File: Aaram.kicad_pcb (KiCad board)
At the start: 2 copper layers, 100 x 100 mm, 52 parts, among them J1 Conn_01x03, J2 Conn_01x02, J3 AC_OUT, J4 SWITCH_IN, J5 5V_OUT, J6 PSU_AC_IN, J8 SPARE_PINS, K1 10A cube relay, K2 10A cube relay, K3 10A cube relay, Q1 BT136-600, Q2 2N2222A, Q3 2N2222A, Q4 2N2222A, U1 ESP32-DevKitC, U2 TLP281-4GB_F_

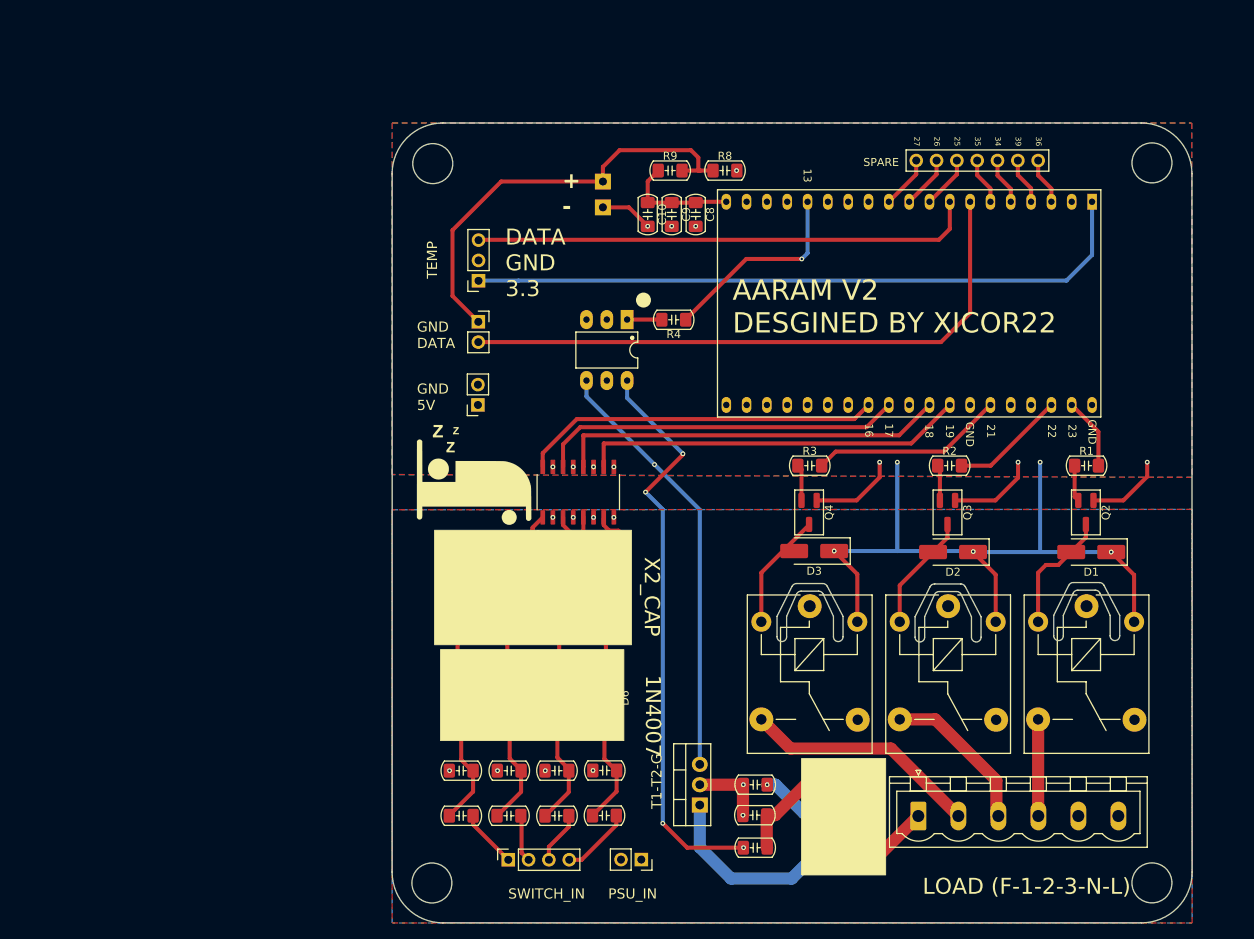
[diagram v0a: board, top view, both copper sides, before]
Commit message: Updated mostly everything
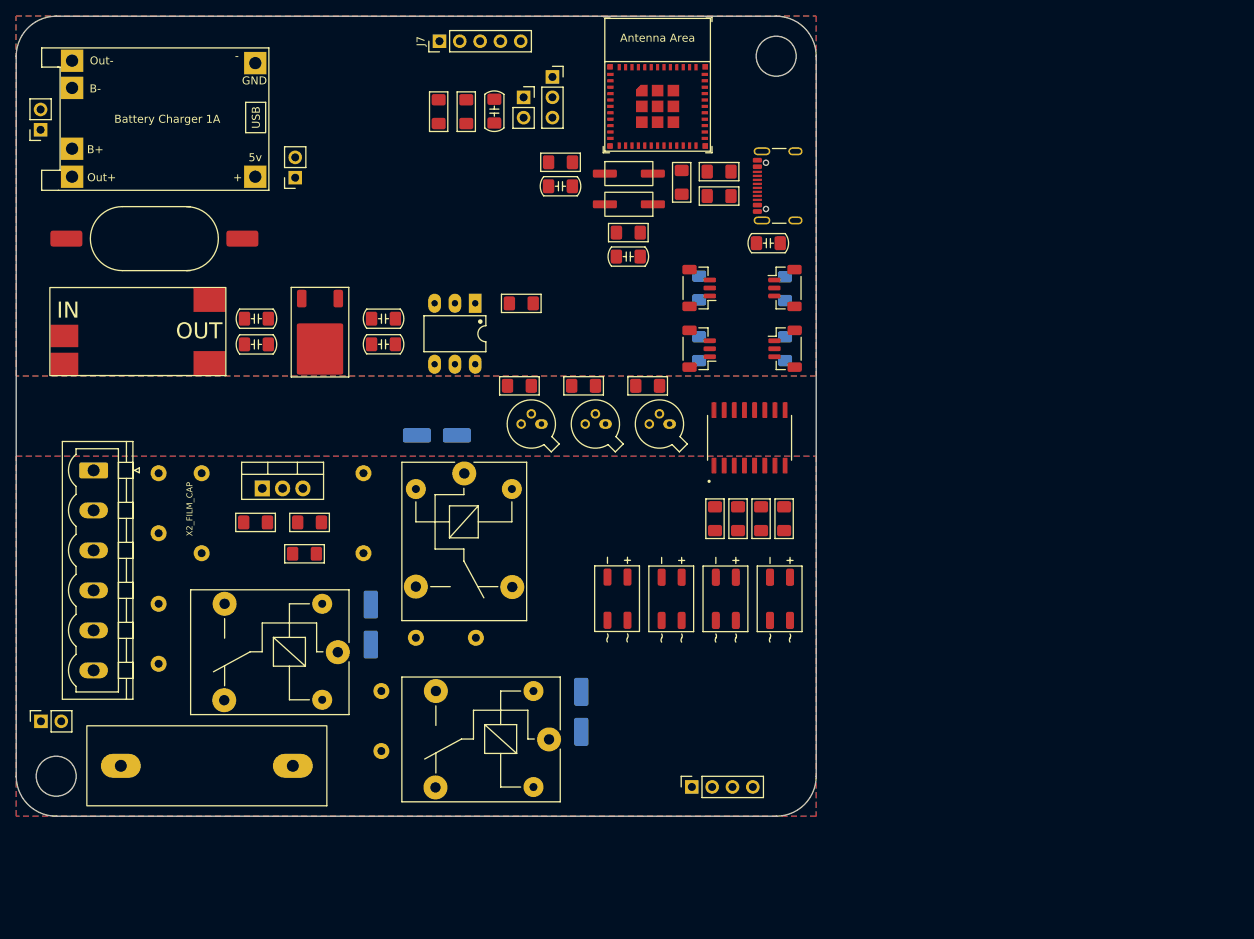
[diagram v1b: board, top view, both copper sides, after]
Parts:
- removed C10, C8, C9: 22uf, PCM_Capacitor_SMD_Handsoldering_AKL:C_1206_3216Metric_Pad1.42x1.75mm
- removed C3, C5: CP_Axial_L10.0mm_D4.5mm_P15.00mm, Xicor_Custom stuff:Axial_Capacitor_P10mm_W4.5mm
- removed D4, D5, D6, D7: 1N4007, Diode_SMD:D_SMA_Handsoldering
- removed G***: LOGO, LOGO
- removed R11, R13: 10K, PCM_Capacitor_SMD_Handsoldering_AKL:C_1206_3216Metric_Pad1.42x1.75mm
- removed R16: 1M, PCM_Capacitor_SMD_Handsoldering_AKL:C_1206_3216Metric_Pad1.42x1.75mm
- added C11: 10uf, PCM_Capacitor_SMD_Handsoldering_AKL:C_1206_3216Metric_Pad1.42x1.75mm, F.Cu at (65.6, 57.4)
- added C12: 10uf, PCM_Capacitor_SMD_Handsoldering_AKL:C_1206_3216Metric_Pad1.42x1.75mm, F.Cu at (65.6, 60.6)
- added C16: 1uf, PCM_Capacitor_SMD_Handsoldering_AKL:C_1206_3216Metric_Pad1.42x1.75mm, F.Cu at (113.7, 47.9)
- added C18: 0.1uf, PCM_Capacitor_SMD_Handsoldering_AKL:C_1206_3216Metric_Pad1.42x1.75mm, F.Cu at (87.7, 40.8)
- added C19: 0.1uf, PCM_Capacitor_SMD_Handsoldering_AKL:C_1206_3216Metric_Pad1.42x1.75mm, F.Cu at (96.2, 49.6)
- added D10: MB6S, PCM_Diode_SMD_AKL:Diode_Bridge_MBS, F.Cu at (108.4, 92.4)
- added D11: MB6S, PCM_Diode_SMD_AKL:Diode_Bridge_MBS, F.Cu at (115.1, 92.4)
- added D8: MB6S, PCM_Diode_SMD_AKL:Diode_Bridge_MBS, F.Cu at (94.8, 92.4)
- added D9: MB6S, PCM_Diode_SMD_AKL:Diode_Bridge_MBS, F.Cu at (101.6, 92.4)
- added F1: Fuse, Xicor_Custom stuff:BLX-A, F.Cu at (43.5, 113.3)
- added J10: Conn_01x03_Socket, Connector_JST:JST_SH_BM03B-SRSS-TB_1x03-1MP_P1.00mm_Vertical, F.Cu at (115.8, 61.1)
- added J11: Conn_01x03_Socket, Connector_JST:JST_SH_BM03B-SRSS-TB_1x03-1MP_P1.00mm_Vertical, F.Cu at (105.1, 61.1)
- added J12: Conn_01x03_Socket, Connector_JST:JST_SH_BM03B-SRSS-TB_1x03-1MP_P1.00mm_Vertical, F.Cu at (105.1, 53.5)
- added J13: Conn_01x03_Socket, Connector_JST:JST_SH_BM03B-SRSS-TB_1x03-1MP_P1.00mm_Vertical, F.Cu at (115.8, 53.5)
- added J7: Conn_01x05, Connector_PinHeader_2.54mm:PinHeader_1x05_P2.54mm_Vertical, F.Cu at (72.6, 22.7)
- added J9: Conn_01x02, Connector_PinSocket_2.54mm:PinSocket_1x02_P2.54mm_Vertical, F.Cu at (22.8, 33.8)
- added R19: 100K, PCM_Resistor_SMD_AKL:R_1206_3216Metric_Pad1.42x1.75mm_HandSolder, F.Cu at (115.7, 82.4)
- added R20: 10K, PCM_Resistor_SMD_AKL:R_1206_3216Metric_Pad1.42x1.75mm_HandSolder, B.Cu at (115.8, 53.6)
- added R21: 10k, PCM_Resistor_SMD_AKL:R_1206_3216Metric_Pad1.42x1.75mm_HandSolder, F.Cu at (96.2, 46.6)
- added R22: 10k, PCM_Resistor_SMD_AKL:R_1206_3216Metric_Pad1.42x1.75mm_HandSolder, F.Cu at (102.9, 40.3)
- added R23: 100K, PCM_Resistor_SMD_AKL:R_1206_3216Metric_Pad1.42x1.75mm_HandSolder, F.Cu at (107.1, 82.4)
- added R25: 10K, PCM_Resistor_SMD_AKL:R_1206_3216Metric_Pad1.42x1.75mm_HandSolder, B.Cu at (105.1, 53.5)
- added R26: 10K, PCM_Resistor_SMD_AKL:R_1206_3216Metric_Pad1.42x1.75mm_HandSolder, B.Cu at (105.1, 61.1)
- added R27: 10K, PCM_Resistor_SMD_AKL:R_1206_3216Metric_Pad1.42x1.75mm_HandSolder, B.Cu at (115.8, 61.1)
- added RV1: Varistor, Xicor_Custom stuff:Varistor_10D431K, F.Cu at (37.5, 93.0)
- added RV2: Varistor, Xicor_Custom stuff:Varistor_10D431K, F.Cu at (69.7, 97.3)
- added RV3: Varistor, Xicor_Custom stuff:Varistor_10D431K, F.Cu at (65.4, 103.9)
- added RV4: Varistor, Xicor_Custom stuff:Varistor_10D431K, F.Cu at (37.5, 84.2)
- added SW1: SW_Push, Xicor_Custom stuff:Tactile switch 6x3, F.Cu at (93.2, 40.8)
- added SW2: SW_Push, Xicor_Custom stuff:SMD Tactile switch, F.Cu at (37.1, 56.1)
- added SW4: SW_Push, Xicor_Custom stuff:Tactile switch 6x3, F.Cu at (99.3, 41.5)
- added U3: ~, Xicor_Custom stuff:Mini_Boost, F.Cu at (34.9, 58.8)
- added U4: ~, Xicor_Custom stuff:TP4056-18650, F.Cu at (51.3, 41.3)
- added U5: TLP281-4GB_F_, Xicor_Custom stuff:SOP127P780X200-16N, F.Cu at (111.4, 72.3)
- C2: footprint Xicor_Custom stuff:Film_Cap_13x13mm_P5.00mm -> PCM_Capacitor_SMD_Handsoldering_AKL:C_1206_3216Metric_Pad1.42x1.75mm
- C6, C7: value CP_Axial_L10.0mm_D4.5mm_P15.00mm -> 10uf; footprint Xicor_Custom stuff:Axial_Capacitor_P10mm_W4.5mm -> PCM_Capacitor_SMD_Handsoldering_AKL:C_1206_3216Metric_Pad1.42x1.75mm
- D1, D2, D3: moved to B.Cu
- J5: value 5V_OUT -> PSU_5V_OUT
- J8: value SPARE_PINS -> USB_C_Receptacle_USB2.0_16P; footprint Connector_PinHeader_2.54mm:PinHeader_1x08_P2.54mm_Vertical -> Connector_USB:USB_C_Receptacle_GCT_USB4105-xx-A_16P_TopMnt_Horizontal
- Q2, Q3, Q4: footprint PCM_Package_TO_SOT_SMD_AKL:SOT-23_BigPads -> PCM_Package_TO_SOT_THT_AKL:TO-18-3_EBC
- R1, R2, R3, R4, R5, R6, R7, R8, R9: footprint PCM_Capacitor_SMD_Handsoldering_AKL:C_1206_3216Metric_Pad1.42x1.75mm -> PCM_Resistor_SMD_AKL:R_1206_3216Metric_Pad1.42x1.75mm_HandSolder
- R10: value 1M -> 10k; footprint PCM_Capacitor_SMD_Handsoldering_AKL:C_1206_3216Metric_Pad1.42x1.75mm -> PCM_Resistor_SMD_AKL:R_1206_3216Metric_Pad1.42x1.75mm_HandSolder
- R12, R14: value 1M -> 5.1k; footprint PCM_Capacitor_SMD_Handsoldering_AKL:C_1206_3216Metric_Pad1.42x1.75mm -> PCM_Resistor_SMD_AKL:R_1206_3216Metric_Pad1.42x1.75mm_HandSolder
- R15, R17: value 10K -> 100K; footprint PCM_Capacitor_SMD_Handsoldering_AKL:C_1206_3216Metric_Pad1.42x1.75mm -> PCM_Resistor_SMD_AKL:R_1206_3216Metric_Pad1.42x1.75mm_HandSolder
- U1: value ESP32-DevKitC -> ESP32-C6-MINI-1/U; footprint Xicor_Custom stuff:ESP32_38Pin -> PCM_Espressif:ESP32-C6-MINI-1
- U2: value TLP281-4GB_F_ -> AZ1117D-3.3TRE1; footprint Xicor_Custom stuff:SOIC127P700X210-16N -> PCM_Package_TO_SOT_SMD_AKL:TO-252-2
- moved J3 111.8 mm to (29.4, 76.3), turned to -90 degrees
- moved K1 93.8 mm to (59.9, 99.1), turned to 180 degrees
- moved D1 90.5 mm to (64.0, 95.6), turned to -90 degrees
- moved R10 82.6 mm to (87.8, 37.8)
- moved R12 81.8 mm to (107.6, 42.0)
- moved R14 81.8 mm to (107.6, 39.0)
- moved C1 81.4 mm to (42.9, 86.7), turned to 90 degrees
- moved J6 77.0 mm to (22.8, 107.7), turned to 90 degrees
- moved R7 72.3 mm to (49.6, 82.8)
- moved R6 69.0 mm to (56.4, 82.8), turned to 0 degrees
- moved C4 68.6 mm to (63.1, 86.7), turned to 90 degrees
- moved Q1 67.5 mm to (50.5, 78.6), turned to 0 degrees
- moved D2 66.1 mm to (72.3, 72.0)
- moved R1 63.7 mm to (90.6, 65.8), turned to 180 degrees
- moved R5 63.3 mm to (55.7, 86.8), turned to 0 degrees
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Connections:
- C6 pad 1: Net-(D6-K) -> GND
- C6 pad 2: AC_N -> +5V
- C7 pad 1: Net-(D7-K) -> GND
- C7 pad 2: AC_N -> +5V
- J1 pad 3: S1_Pin -> Sensor 1
- J2 pad 2: S2_Pin -> Sensor 2
- J3 pad 2: LOAD_1 -> LOAD_2
- J3 pad 3: LOAD_2 -> LOAD_1
- J3 pad 6: AC_L -> Net-(J3-Pin_6)
- J4 pad 1: S1 -> AC_IN_1
- J4 pad 2: S2 -> AC_IN_2
- J4 pad 3: S3 -> AC_IN_3
- J4 pad 4: S4 -> AC_IN_4
- J5 pad 1: +5V -> PSU_5V
- Q2 pad 3: Net-(D1-A) -> Net-(D2-A)
- Q3 pad 3: Net-(D2-A) -> Net-(D3-A)
- Q4 pad 3: Net-(D3-A) -> Net-(D1-A)
- R1 pad 2: D3 -> D2
- R10 pad 1: Net-(D4-A) -> +3.3V
- R10 pad 2: S1 -> Net-(U1-EN/CHIP_PU)
- R12 pad 1: Net-(D5-A) -> GND
- R12 pad 2: S2 -> Net-(J8-CC1)
- R14 pad 1: Net-(D6-A) -> GND
- R14 pad 2: S4 -> Net-(J8-CC2)
- R15 pad 1: AC_N -> Net-(U5-A2)
- R15 pad 2: Net-(D6-A) -> Net-(D9-+)
- R17 pad 1: AC_N -> Net-(U5-A3)
- R2 pad 2: D2 -> D1
- R3 pad 2: D1 -> D3
- U1 pad 1: +3.3V -> GND
- U1 pad 10: SP3 -> SP5
- U1 pad 11: SP2 -> GND
- U1 pad 13: unconnected-(U1-MTDI/GPIO12/ADC2_CH5-Pad13) -> SP1
- U1 pad 15: T1_Pin -> Sensor 1
- U1 pad 16: unconnected-(U1-SD_DATA2/GPIO9-Pad16) -> Sensor 2
- U1 pad 17: unconnected-(U1-SD_DATA3/GPIO10-Pad17) -> USB-
- U1 pad 18: unconnected-(U1-CMD-Pad18) -> USB+
- U1 pad 19: +5V -> AC_IN_1
- U1 pad 2: unconnected-(U1-CHIP_PU-Pad2) -> GND
- U1 pad 20: unconnected-(U1-SD_CLK/GPIO6-Pad20) -> AC_IN_2
- U1 pad 22: unconnected-(U1-SD_DATA1/GPIO8-Pad22) -> Net-(U1-GPIO8)
- U1 pad 23: unconnected-(U1-MTDO/GPIO15/ADC2_CH3-Pad23) -> Net-(U1-GPIO9)
- U1 pad 24: unconnected-(U1-ADC2_CH2/GPIO2-Pad24) -> AC_IN_3
- U1 pad 25: unconnected-(U1-GPIO0/BOOT/ADC2_CH1-Pad25) -> AC_IN_4
- U1 pad 26: unconnected-(U1-ADC2_CH0/GPIO4-Pad26) -> D3
- U1 pad 27: O1 -> D2
- U1 pad 28: O2 -> D1
- U1 pad 29: unconnected-(U1-GPIO5-Pad29) -> T1_Pin
- U1 pad 3: SP8 -> +3.3V
- U1 pad 30: O3 -> unconnected-(U1-U0RXD/GPIO17-Pad30)
- U1 pad 31: O4 -> unconnected-(U1-U0TXD/GPIO16-Pad31)
- U1 pad 32: GND -> unconnected-(U1-NC-Pad32)
- U1 pad 33: D1 -> unconnected-(U1-NC-Pad33)
- U1 pad 36: D2 -> GND
- U1 pad 37: D3 -> GND
- U1 pad 4: SP7 -> unconnected-(U1-NC-Pad4)
- U1 pad 5: SP6 -> SP2
- U1 pad 6: SP5 -> SP3
- U1 pad 7: S2_Pin -> unconnected-(U1-NC-Pad7)
- U1 pad 8: S1_Pin -> Net-(U1-EN/CHIP_PU)
- U2 pad 1: Net-(D4-K) -> GND
- U2 pad 2: AC_N -> +3.3V
- U2 pad 3: Net-(D5-K) -> +5V
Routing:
- net +5V: track 101.3 -> 0.00 mm, vias 5 -> 0
- net +3.3V: track 84.6 -> 0.00 mm
- net S2_Pin: track 76.9 -> 0.00 mm
- net Net-(OC1-Pad6): track 72.4 -> 0.00 mm, vias 4 -> 0
- net S1_Pin: track 62.8 -> 0.00 mm
- net Net-(J2-Pin_1): track 54.7 -> 0.00 mm
- net Net-(Q1-G): track 53.8 -> 0.00 mm, vias 1 -> 0
- net O3: track 48.8 -> 0.00 mm
- net O4: track 48.2 -> 0.00 mm
- net O2: track 45.6 -> 0.00 mm
- net O1: track 44.9 -> 0.00 mm
- net GND: track 39.0 -> 0.00 mm, vias 11 -> 0
- net LOAD_F: track 37.5 -> 0.00 mm
- net LOAD_1: track 29.6 -> 0.00 mm
- net T1_Pin: track 25.1 -> 0.00 mm, vias 1 -> 0
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- added copper zone on B.Cu, net +5V
- added copper zone on F.Cu, net GND
- removed copper zone on F.Cu, net +5V
- removed copper zone on B.Cu, net GND
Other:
- outline, holes or cut-outs redrawn
- board text removed: "+ -"
- board text removed: "1N4007"
- board text removed: "AARAM V2 DESGINED BY XICOR22"
- board text removed: "CURRENT"
- board text removed: "DATA GND 3.3"
- board text removed: "GND 5V"
- board text removed: "GND DATA"
- board text removed: "LOAD (F-1-2-3-N-L)"
- board text removed: "PSU_IN"
- board text removed: "SPARE"
- board text removed: "SWITCH_IN"
- board text removed: "T1-T2-G"
- board text removed: "TEMP"
- board text removed: "X2_CAP"
